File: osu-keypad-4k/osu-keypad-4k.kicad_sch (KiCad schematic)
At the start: 14 parts

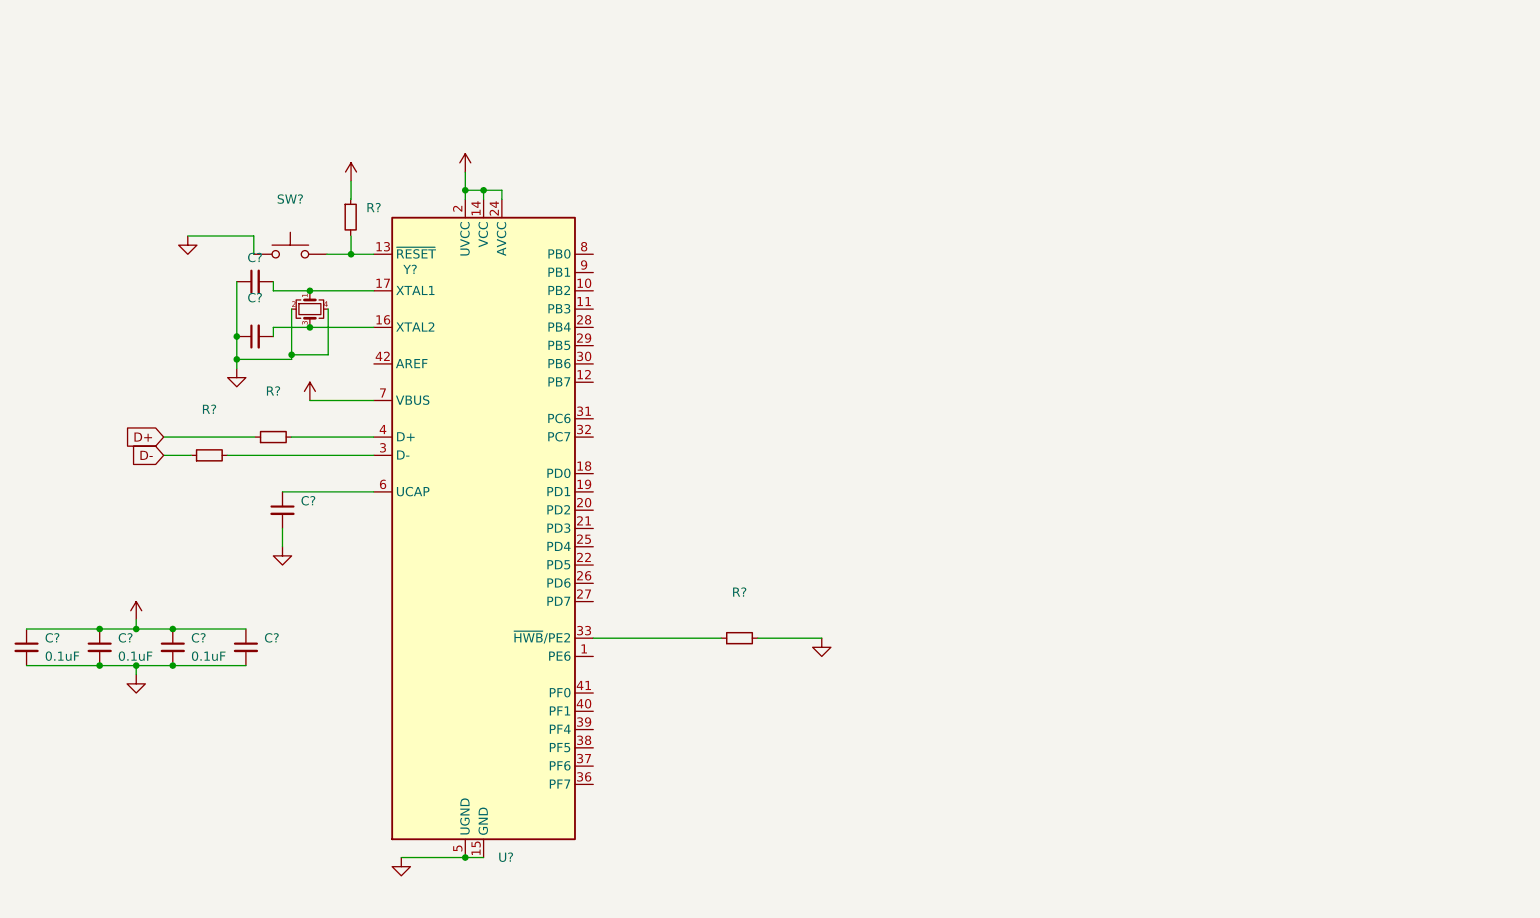
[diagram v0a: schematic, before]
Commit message: Finish Schematic
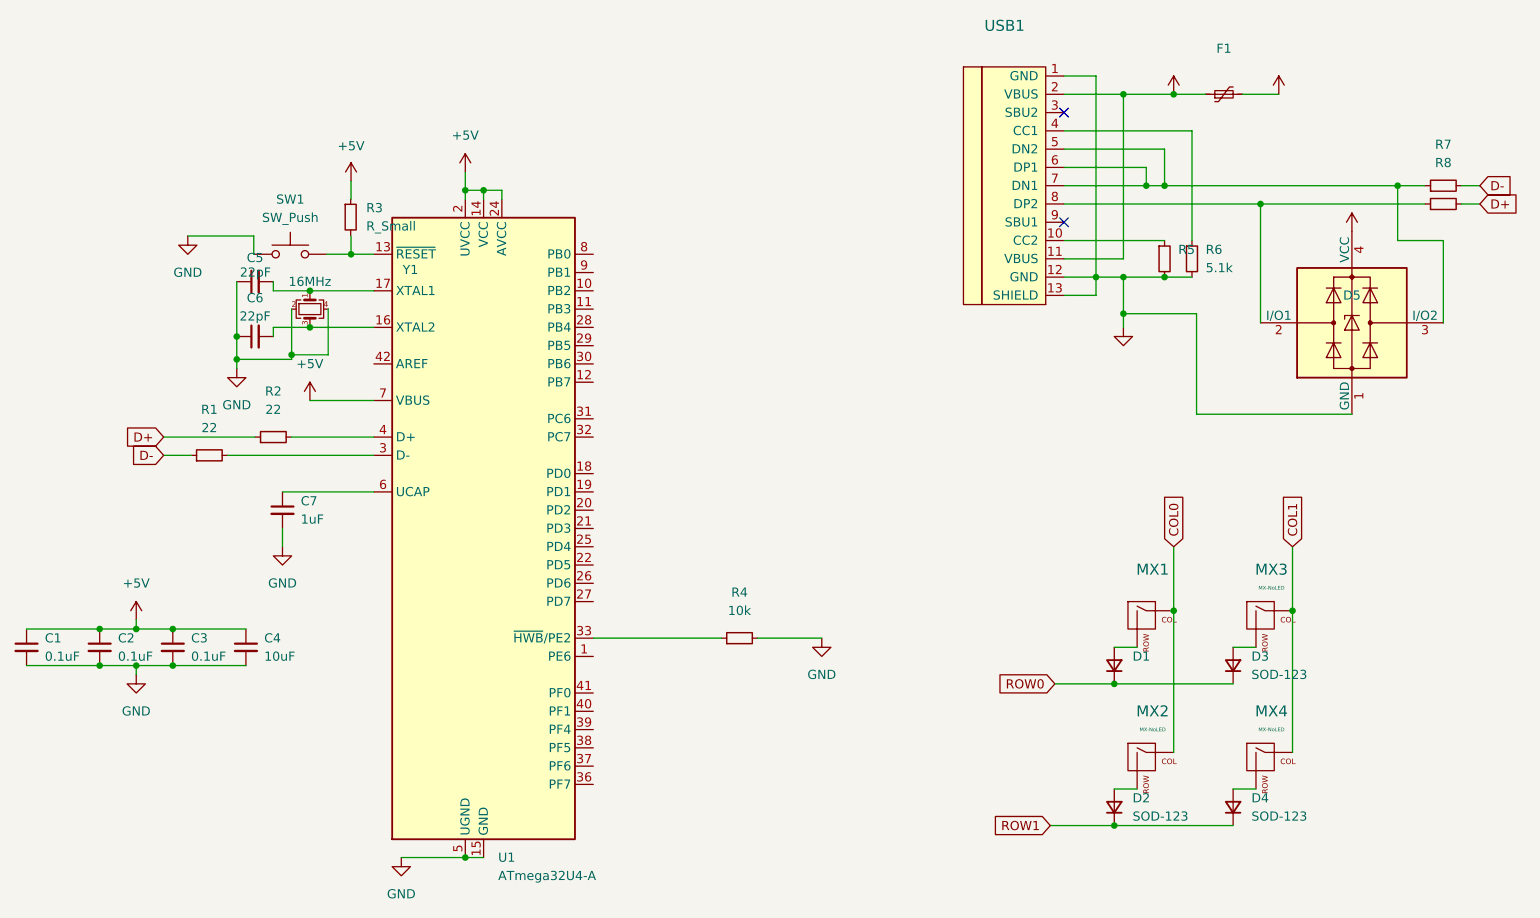
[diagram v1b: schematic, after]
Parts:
- added D1: (no value), symbol Device:D_Small
- added D2, D3, D4: SOD-123, symbol Device:D_Small
- added D5: (no value), symbol Power_Protection:PRTR5V0U2X
- added F1: (no value), symbol Device:Polyfuse_Small
- added MX1: (no value), symbol MX_Alps_Hybrid:MX-NoLED
- added MX2, MX3, MX4: MX-NoLED, symbol MX_Alps_Hybrid:MX-NoLED
- added R5, R7, R8: (no value), symbol Device:R_Small
- added R6: 5.1k, symbol Device:R_Small
- added USB1: (no value), symbol Type-C:HRO-TYPE-C-31-M-12
- C4: renamed from C?; value (none) -> 10uF
- C5, C6: renamed from C?; value (none) -> 22pF
- C7: renamed from C?; value (none) -> 1uF
- R1, R2: renamed from R?; value (none) -> 22
- R3: renamed from R?; value (none) -> R_Small
- R4: renamed from R?; value (none) -> 10k
- SW1: renamed from SW?; value (none) -> SW_Push
- U1: renamed from U?; value (none) -> ATmega32U4-A; footprint (none) -> Package_QFP:TQFP-44_10x10mm_P0.8mm
- Y1: renamed from Y?; value (none) -> 16MHz
- gave numbers to parts that had none: 3
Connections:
- net +5V: now also F1.2
- net D+: now also R8.2
- net D-: now also R7.2
- net GND: now also D5.1 (GND), R5.2, R6.2, USB1.1 (GND), USB1.12 (GND), USB1.13 (SHIELD)
- new net: D5.2 (I/O1), R8.1, USB1.8 (DP2)
- new net: D4.2 (A), MX4.2 (ROW)
- new net: R6.1, USB1.4 (CC1)
- new net: D5.3 (I/O2), R7.1, USB1.5 (DN2), USB1.6 (DP1), USB1.7 (DN1)
- new net: D3.2 (A), MX3.2 (ROW)
- new net: D1.2 (A), MX1.2 (ROW)
- new net: R5.1, USB1.10 (CC2)
- new net: D2.2 (A), MX2.2 (ROW)
- new net COL0: MX1.1 (COL), MX2.1 (COL)
- new net COL1: MX3.1 (COL), MX4.1 (COL)
- new net ROW0: D1.1 (K), D3.1 (K)
- new net ROW1: D2.1 (K), D4.1 (K)
- new net VCC: D5.4 (VCC), F1.1, USB1.11 (VBUS), USB1.2 (VBUS)
- no-connect marks 0 -> 2

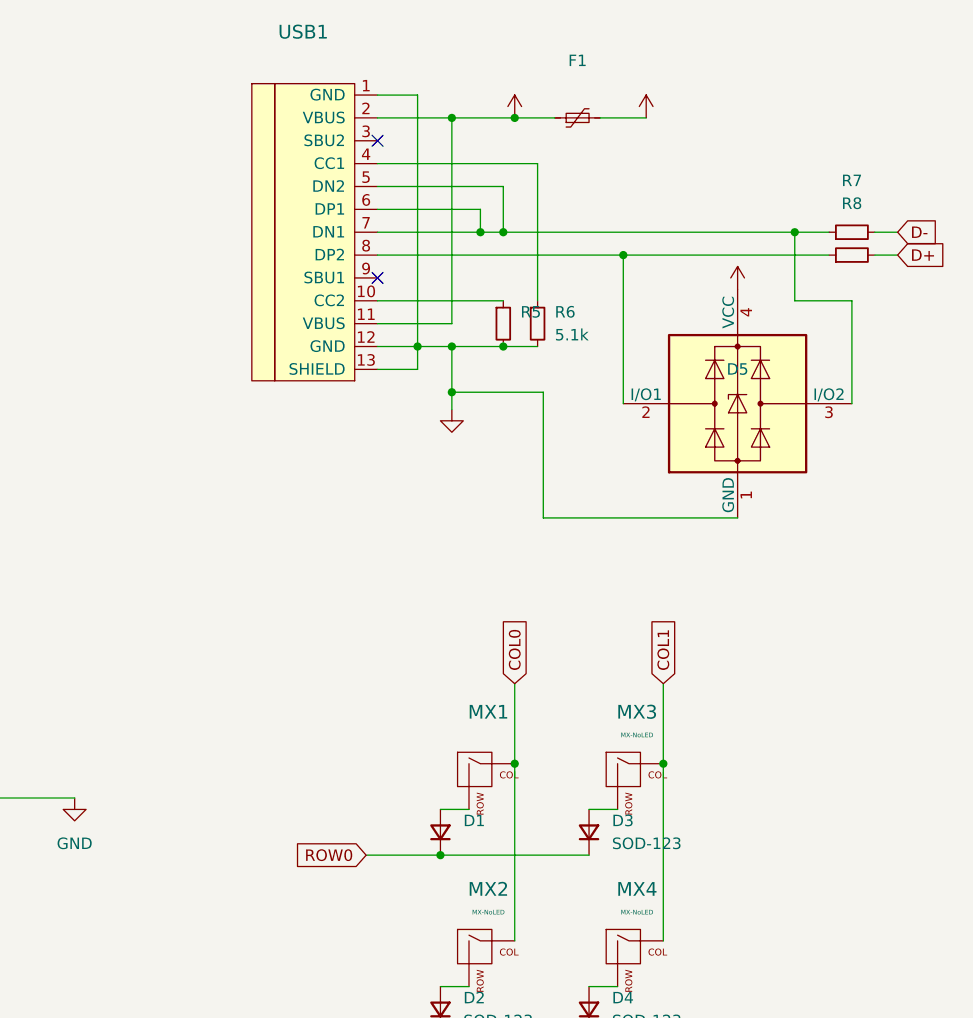
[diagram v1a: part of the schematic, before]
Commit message: start pcb
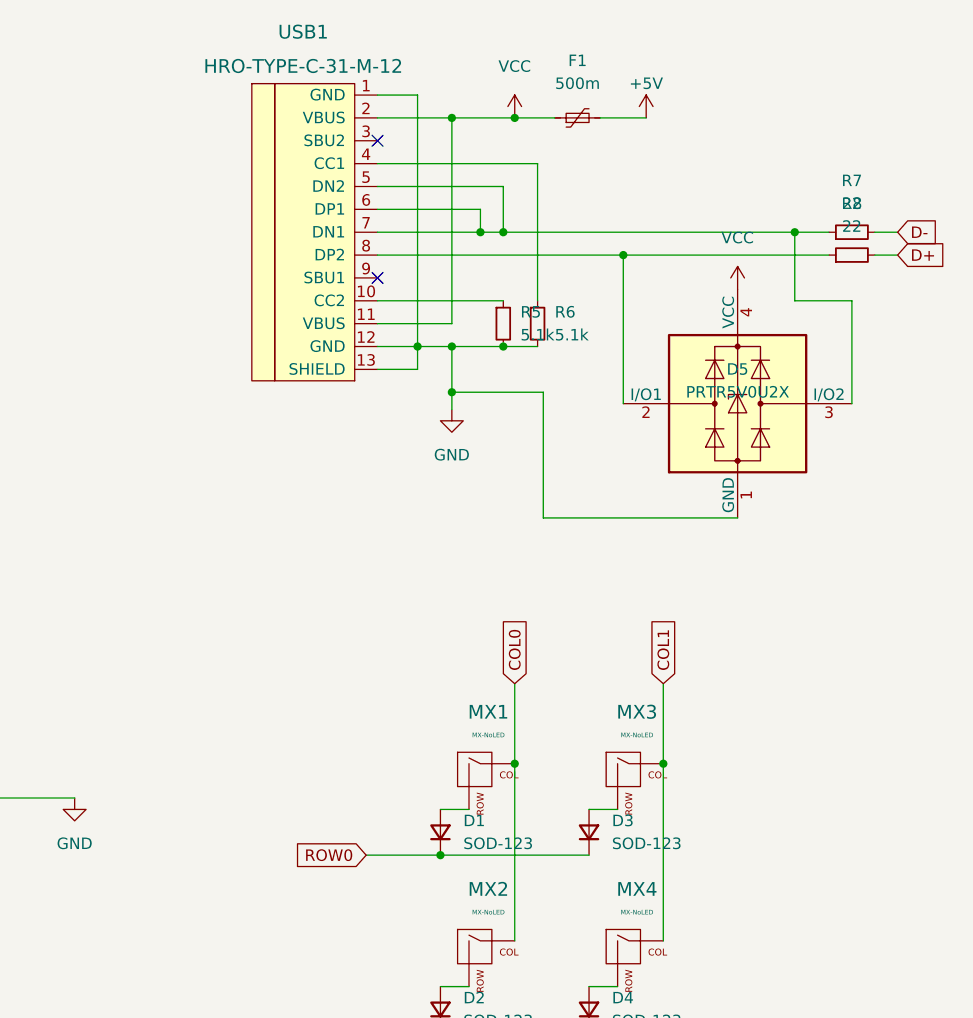
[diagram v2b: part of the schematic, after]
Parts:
- C1, C2, C3, C4, C5, C6, C7: footprint (none) -> Capacitor_SMD:C_0805_2012Metric
- D1: value (none) -> SOD-123; footprint (none) -> Diode_SMD:D_SOD-123
- D2, D3, D4: footprint (none) -> Diode_SMD:D_SOD-123
- D5: value (none) -> PRTR5V0U2X; footprint (none) -> Package_TO_SOT_SMD:SOT-143
- F1: value (none) -> 500m; footprint (none) -> Fuse:Fuse_1206_3216Metric
- MX1: value (none) -> MX-NoLED; footprint (none) -> MX_Alps_Hybrid:MX-1U-NoLED
- MX2, MX3, MX4: footprint (none) -> MX_Alps_Hybrid:MX-1U-NoLED
- R1, R2, R3, R4, R6: footprint (none) -> Resistor_SMD:R_0805_2012Metric
- R5: value (none) -> 5.1k; footprint (none) -> Resistor_SMD:R_0805_2012Metric
- R7, R8: value (none) -> 22; footprint (none) -> Resistor_SMD:R_0805_2012Metric
- SW1: footprint (none) -> random-keyboard-parts:SKQG-1155865
- USB1: value (none) -> HRO-TYPE-C-31-M-12; footprint (none) -> Type-C:HRO-TYPE-C-31-M-12
- Y1: footprint (none) -> Crystal:Crystal_SMD_3225-4Pin_3.2x2.5mm

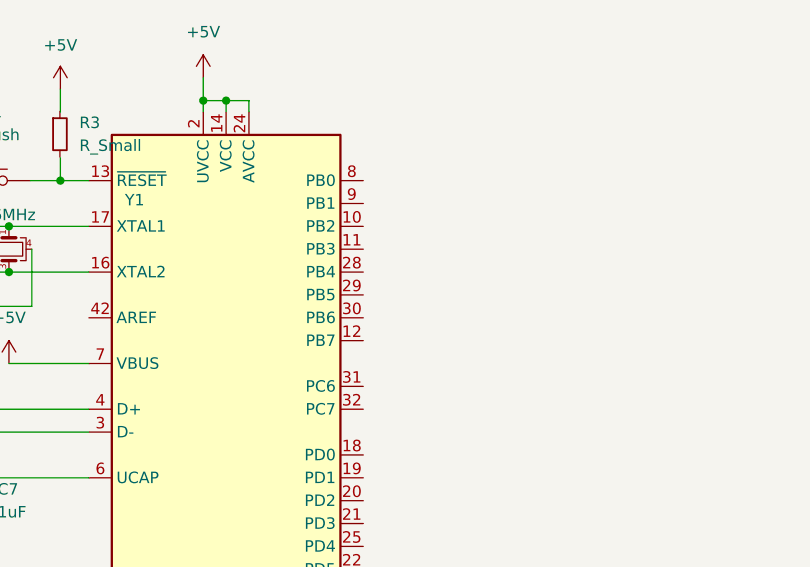
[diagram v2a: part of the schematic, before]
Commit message: pcb
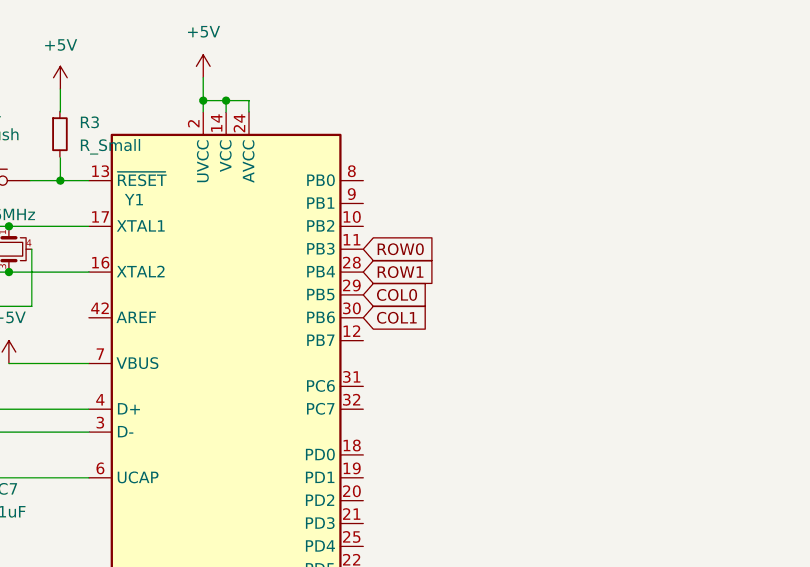
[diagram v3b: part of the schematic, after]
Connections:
- net COL0: now also U1.29 (PB5)
- net COL1: now also U1.30 (PB6)
- net ROW0: now also U1.11 (PB3)
- net ROW1: now also U1.28 (PB4)
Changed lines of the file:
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@@
+    )
+  )
+  (global_label "ROW1" (shape input) (at 116.84 64.77 0) (fields_autoplaced)
+    (effects (font (size 1.27 1.27)) (justify left))
+    (property "Intersheet References" "${INTERSHEET_REFS}" (id 0) (at 124.5145 64.6906 0)
+      (effects (font (size 1.27 1.27)) (justify left) hide)
     )
   )
@@
     )
   )
+  (global_label "COL1" (shape input) (at 116.84 69.85 0) (fields_autoplaced)
+    (effects (font (size 1.27 1.27)) (justify left))
+    (property "Intersheet References" "${INTERSHEET_REFS}" (id 0) (at 124.0912 69.7706 0)
+      (effects (font (size 1.27 1.27)) (justify left) hide)
+    )
+  )
   (global_label "D-" (shape input) (at 240.03 45.085 0) (fields_autoplaced)
     (effects (font (size 1.27 1.27)) (justify left))
     (property "Intersheet References" "${INTERSHEET_REFS}" (id 0) (at 245.2855 45.0056 0)
+      (effects (font (size 1.27 1.27)) (justify left) hide)
+    )
+  )
+  (global_label "ROW0" (shape input) (at 116.84 62.23 0) (fields_autoplaced)
+    (effects (font (size 1.27 1.27)) (justify left))
+    (property "Intersheet References" "${INTERSHEET_REFS}" (id 0) (at 124.5145 62.1506 0)
       (effects (font (size 1.27 1.27)) (justify left) hide)
     )
@@
       (effects (font (size 1.27 1.27)) (justify left) hide)
     )
+  )
+  (global_label "COL0" (shape input) (at 116.84 67.31 0) (fields_autoplaced)
+    (effects (font (size 1.27 1.27)) (justify left))
+    (property "Intersheet References" "${INTERSHEET_REFS}" (id 0) (at 124.0912 67.2306 0)
+      (effects (font (size 1.27 1.27)) (justify left) hide)
+    )
